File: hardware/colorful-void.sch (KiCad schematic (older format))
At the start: 4 parts, among them J1 Raspberry_Pi_Zero, J2 Barrel_Jack, J3 Conn_01x03, U1 74AHCT125

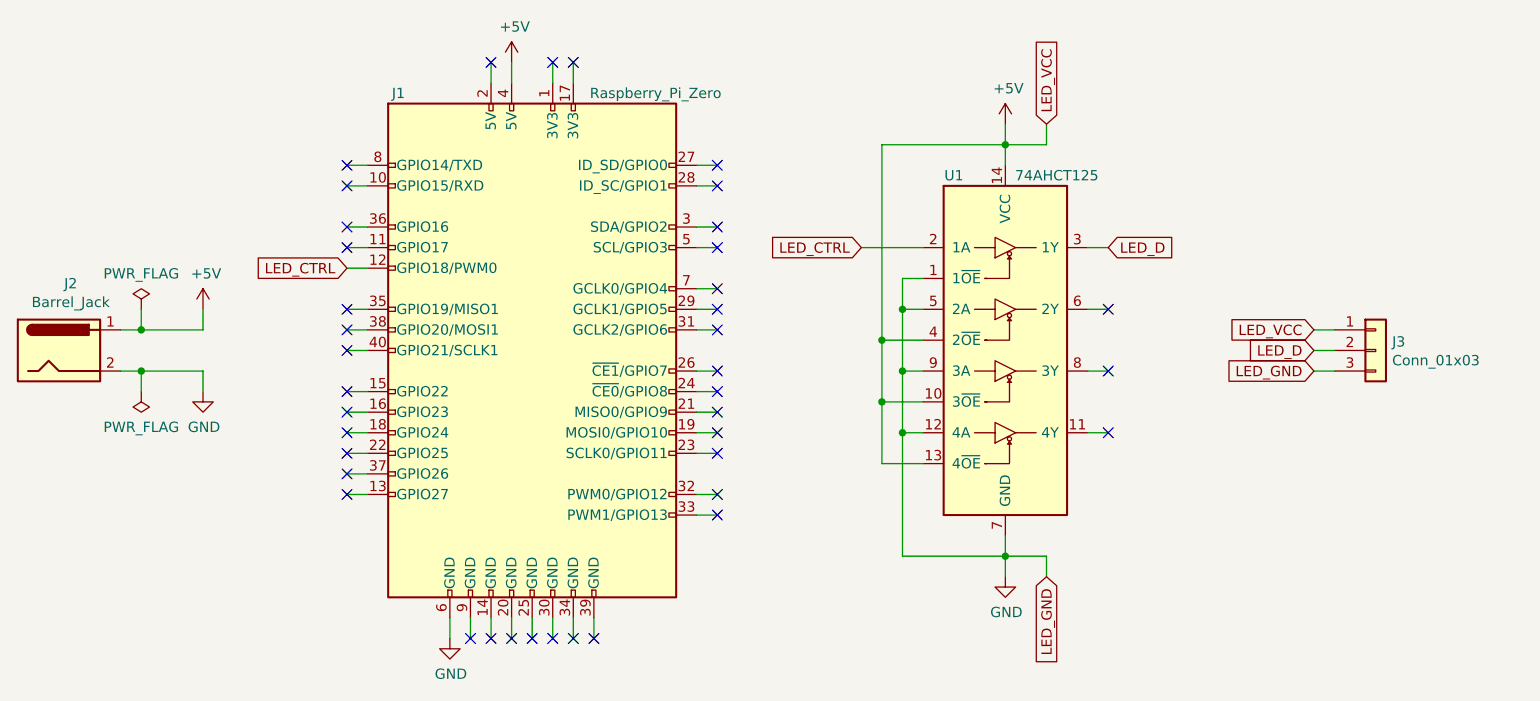
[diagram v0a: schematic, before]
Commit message: PCB rev. 1
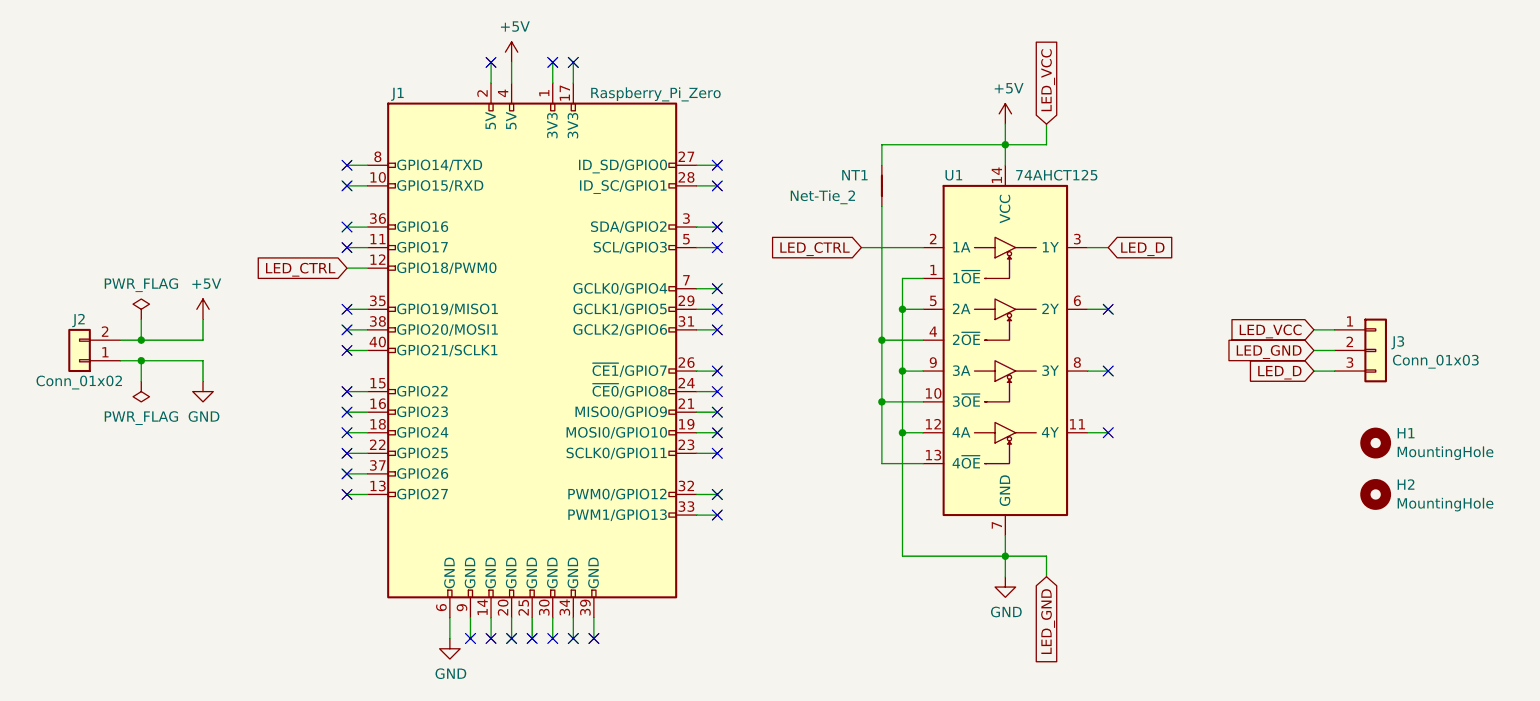
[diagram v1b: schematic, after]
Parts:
- removed J2: Barrel_Jack, symbol Connector:Barrel_Jack
- added H1, H2: MountingHole, misc_hardware:MountingHole_M2.5, symbol Mechanical:MountingHole
- added J2: Conn_01x02, misc_hardware:TerminalBlock_Kaweei_1x02_P2.54mm_Horizontal, symbol Connector_Generic:Conn_01x02
- added NT1: Net-Tie_2, NetTie:NetTie-2_SMD_Pad0.5mm, symbol Device:Net-Tie_2
- J1: footprint (none) -> Connector_PinHeader_2.54mm:PinHeader_2x06_P2.54mm_Vertical
- J3: footprint (none) -> misc_hardware:TerminalBlock_Kaweei_1x03_P2.54mm_Horizontal
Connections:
- net +5V: now also J2.2 (Pin_2), NT1.2; no longer U1.10 (3~OE), U1.13 (4~OE), U1.4 (2~OE)
- net GND: now also J3.2 (Pin_2), J2.1 (Pin_1); no longer J3.3 (Pin_3)
- net LED_D: now also J3.3 (Pin_3); no longer J3.2 (Pin_2)
- new net: NT1.1, U1.10 (3~OE), U1.13 (4~OE), U1.4 (2~OE)
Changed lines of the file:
@@
 F 0 "J1" H 4250 5050 50  0000 C CNN
 F 1 "Raspberry_Pi_Zero" H 5500 5050 50  0000 C CNN
-F 2 "" H 4900 3800 50  0001 C CNN
+F 2 "Connector_PinHeader_2.54mm:PinHeader_2x06_P2.54mm_Vertical" H 4900 3800 50  0001 C CNN
 F 3 "https://www.raspberrypi.org/documentation/hardware/raspberrypi/schematics/rpi_SCH_3bplus_1p0_reduced.pdf" H 4900 3800 50  0001 C CNN
 	1    4900 3800
@@
 	6700 3450 6700 3600
 Wire Wire Line
-	6700 4800 7200 4800
-Wire Wire Line
 	6700 3450 6800 3450
 Connection ~ 6700 3600
@@
 Connection ~ 6600 3750
 Wire Wire Line
-	6600 3750 6600 2800
+	6600 3750 6600 3100
 Connection ~ 6600 4050
 Wire Wire Line
@@
 NoConn ~ 5000 2400
 NoConn ~ 5100 2400
-$Comp
-L Connector:Barrel_Jack J2
-U 1 1 5FDE4F93
-P 2600 3800
-F 0 "J2" H 2657 4125 50  0000 C CNN
-F 1 "Barrel_Jack" H 2657 4034 50  0000 C CNN
-F 2 "" H 2650 3760 50  0001 C CNN
-F 3 "~" H 2650 3760 50  0001 C CNN
-	1    2600 3800
-	1    0    0    -1
-$EndComp
-Wire Wire Line
-	2900 3700 3000 3700
-Wire Wire Line
-	3000 3700 3000 3600
-Wire Wire Line
-	2900 3900 3000 3900
-Wire Wire Line
-	3000 3900 3000 4000
+Wire Wire Line
+	2900 3750 3000 3750
+Wire Wire Line
+	3000 3750 3000 3650
+Wire Wire Line
+	2900 3850 3000 3850
+Wire Wire Line
+	3000 3850 3000 3950
 $Comp
 L power:+5V #PWR03
 U 1 1 5FDEBA13
-P 3300 3600
-F 0 "#PWR03" H 3300 3450 50  0001 C CNN
-F 1 "+5V" H 3315 3773 50  0000 C CNN
-F 2 "" H 3300 3600 50  0001 C CNN
-F 3 "" H 3300 3600 50  0001 C CNN
-	1    3300 3600
+P 3300 3650
+F 0 "#PWR03" H 3300 3500 50  0001 C CNN
+F 1 "+5V" H 3315 3823 50  0000 C CNN
+F 2 "" H 3300 3650 50  0001 C CNN
+F 3 "" H 3300 3650 50  0001 C CNN
+	1    3300 3650
 	1    0    0    -1
 $EndComp
@@
 L power:GND #PWR04
 U 1 1 5FDEC1C7
-P 3300 4000
-F 0 "#PWR04" H 3300 3750 50  0001 C CNN
-F 1 "GND" H 3305 3827 50  0000 C CNN
-F 2 "" H 3300 4000 50  0001 C CNN
-F 3 "" H 3300 4000 50  0001 C CNN
-	1    3300 4000
+P 3300 3950
+F 0 "#PWR04" H 3300 3700 50  0001 C CNN
+F 1 "GND" H 3305 3777 50  0000 C CNN
+F 2 "" H 3300 3950 50  0001 C CNN
+F 3 "" H 3300 3950 50  0001 C CNN
+	1    3300 3950
 	1    0    0    -1
 $EndComp
@@
 L power:PWR_FLAG #FLG01
 U 1 1 5FDF5B6E
-P 3000 3600
-F 0 "#FLG01" H 3000 3675 50  0001 C CNN
-F 1 "PWR_FLAG" H 3000 3773 50  0000 C CNN
-F 2 "" H 3000 3600 50  0001 C CNN
-F 3 "~" H 3000 3600 50  0001 C CNN
-	1    3000 3600
-	1    0    0    -1
-$EndComp
-Wire Wire Line
-	3300 3600 3300 3700
-Wire Wire Line
-	3300 3700 3000 3700
-Connection ~ 3000 3700
-Wire Wire Line
-	3300 4000 3300 3900
-Wire Wire Line
-	3300 3900 3000 3900
-Connection ~ 3000 3900
+P 3000 3650
+F 0 "#FLG01" H 3000 3725 50  0001 C CNN
+F 1 "PWR_FLAG" H 3000 3823 50  0000 C CNN
+F 2 "" H 3000 3650 50  0001 C CNN
+F 3 "~" H 3000 3650 50  0001 C CNN
+	1    3000 3650
+	1    0    0    -1
+$EndComp
+Wire Wire Line
+	3300 3650 3300 3750
+Wire Wire Line
+	3300 3750 3000 3750
+Connection ~ 3000 3750
+Wire Wire Line
+	3300 3950 3300 3850
+Wire Wire Line
+	3300 3850 3000 3850
+Connection ~ 3000 3850
 $Comp
 L power:PWR_FLAG #FLG02
 U 1 1 5FDFB526
-P 3000 4000
-F 0 "#FLG02" H 3000 4075 50  0001 C CNN
-F 1 "PWR_FLAG" H 3000 4173 50  0000 C CNN
-F 2 "" H 3000 4000 50  0001 C CNN
-F 3 "~" H 3000 4000 50  0001 C CNN
-	1    3000 4000
+P 3000 3950
+F 0 "#FLG02" H 3000 4025 50  0001 C CNN
+F 1 "PWR_FLAG" H 3000 4123 50  0000 C CNN
+F 2 "" H 3000 3950 50  0001 C CNN
+F 3 "~" H 3000 3950 50  0001 C CNN
+	1    3000 3950
 	-1   0    0    1
 $EndComp
@@
 F 0 "J3" H 9080 3842 50  0000 L CNN
 F 1 "Conn_01x03" H 9080 3751 50  0000 L CNN
-F 2 "" H 9000 3800 50  0001 C CNN
+F 2 "misc_hardware:TerminalBlock_Kaweei_1x03_P2.54mm_Horizontal" H 9000 3800 50  0001 C CNN
 F 3 "~" H 9000 3800 50  0001 C CNN
 	1    9000 3800
@@
 Text GLabel 8700 3700 0    50   Input ~ 0
 LED_VCC
+Text GLabel 8700 3900 0    50   Input ~ 0
+LED_D
 Text GLabel 8700 3800 0    50   Input ~ 0
-LED_D
-Text GLabel 8700 3900 0    50   Input ~ 0
 LED_GND
 Wire Wire Line
@@
 	6500 3300 6800 3300
 NoConn ~ 4700 2400
+$Comp
+L Connector_Generic:Conn_01x02 J2
+U 1 1 5FEFCA38
+P 2700 3850
+F 0 "J2" H 2700 3650 50  0000 C CNN
+F 1 "Conn_01x02" H 2700 3950 50  0000 C CNN
+F 2 "misc_hardware:TerminalBlock_Kaweei_1x02_P2.54mm_Horizontal" H 2700 3850 50  0001 C CNN
+F 3 "~" H 2700 3850 50  0001 C CNN
+	1    2700 3850
+	-1   0    0    1
+$EndComp
+$Comp
+L Device:Net-Tie_2 NT1
+U 1 1 5FF0F2A7
+P 6600 3000
+F 0 "NT1" V 6650 3200 50  0000 R CNN
+F 1 "Net-Tie_2" V 6550 3450 50  0000 R CNN
+F 2 "NetTie:NetTie-2_SMD_Pad0.5mm" H 6600 3000 50  0001 C CNN
+F 3 "~" H 6600 3000 50  0001 C CNN
+	1    6600 3000
+	0    -1   -1   0
+$EndComp
+Wire Wire Line
+	6600 2900 6600 2800
+Wire Wire Line
+	6700 4800 7200 4800
+$Comp
+L Mechanical:MountingHole H1
+U 1 1 5FF4F0EB
+P 9000 4250
+F 0 "H1" H 9100 4296 50  0000 L CNN
+F 1 "MountingHole" H 9100 4205 50  0000 L CNN
+F 2 "misc_hardware:MountingHole_M2.5" H 9000 4250 50  0001 C CNN
+F 3 "~" H 9000 4250 50  0001 C CNN
+	1    9000 4250
+	1    0    0    -1
+$EndComp
+$Comp
+L Mechanical:MountingHole H2
+U 1 1 5FF5065F
+P 9000 4500
+F 0 "H2" H 9100 4546 50  0000 L CNN
+F 1 "MountingHole" H 9100 4455 50  0000 L CNN
+F 2 "misc_hardware:MountingHole_M2.5" H 9000 4500 50  0001 C CNN
+F 3 "~" H 9000 4500 50  0001 C CNN
+	1    9000 4500
+	1    0    0    -1
+$EndComp
 $EndSCHEMATC
